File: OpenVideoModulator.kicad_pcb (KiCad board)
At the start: 2 copper layers, 38.6 x 24.9 mm, 22 parts, among them J1 CONN_6, J2 S-Video+Composite_Combo, P1 OSHW_LOGO, U1 AD724, Y1 4.433619M

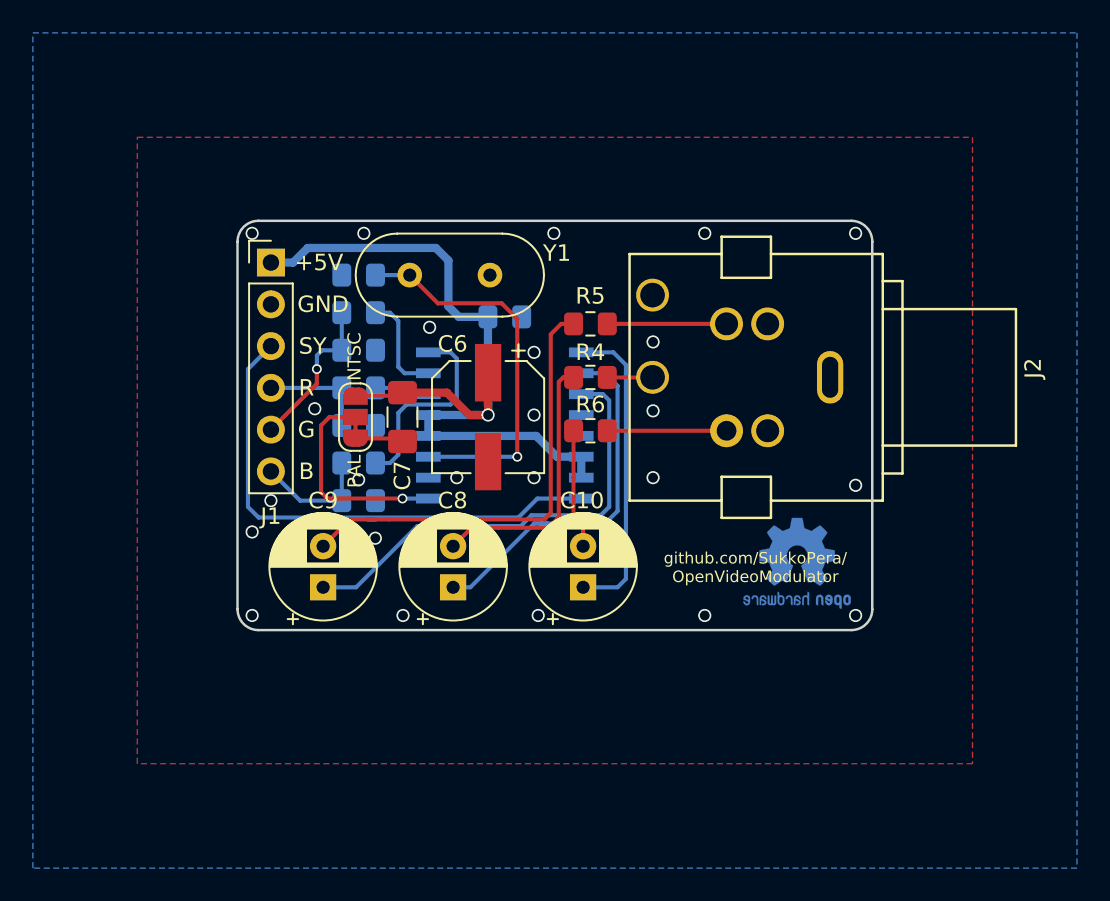
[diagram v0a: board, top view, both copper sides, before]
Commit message: 1st version
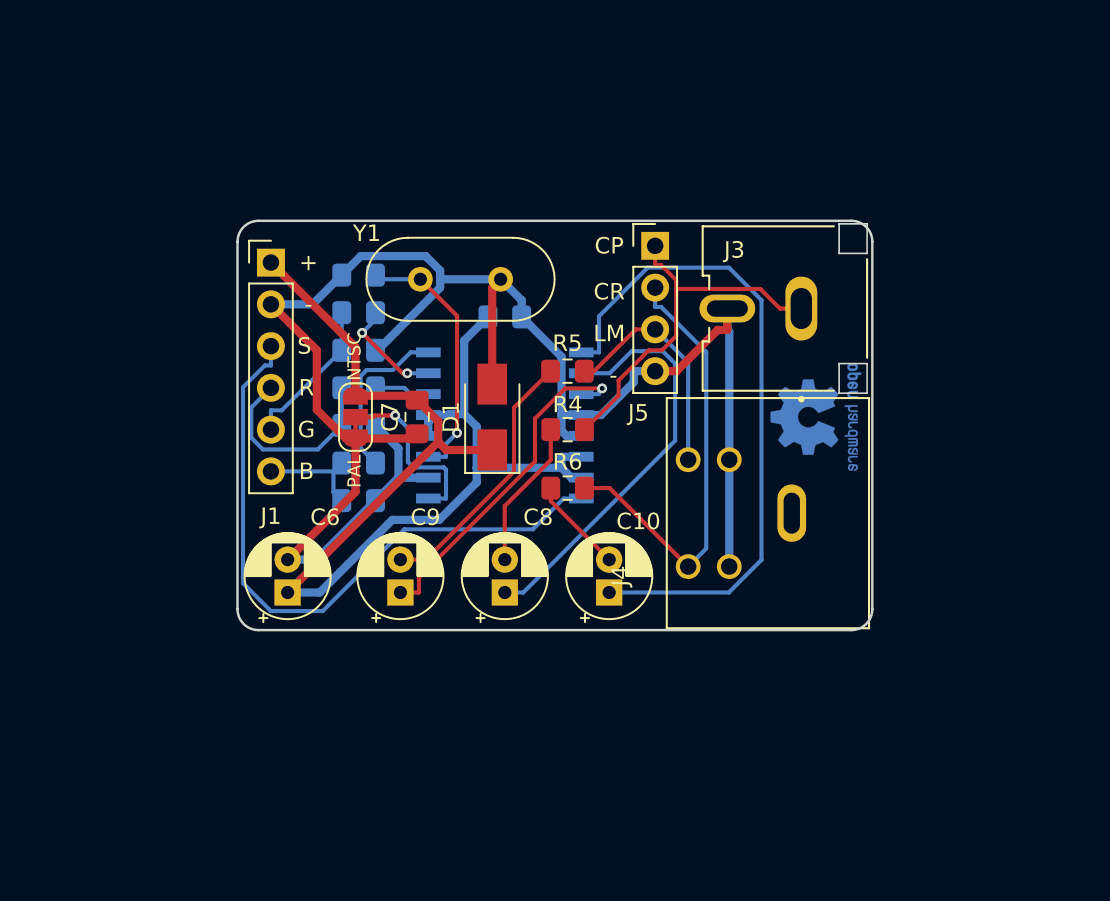
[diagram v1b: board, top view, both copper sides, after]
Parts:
- removed J2: S-Video+Composite_Combo, OpenVideoModulator:AV-MDC-401
- added D1: 1N4001, Diode_SMD:D_SMA, F.Cu at (129.5, 61.5)
- added J3: RCA, OpenVideoModulator:CUI_RCJ-044, F.Cu at (148.3, 54.9)
- added J4: Mini-DIN-4, OpenVideoModulator:CUI_MD-40S_1234, F.Cu at (146.3, 67.3)
- added J5: Conn_01x04_Male, Connector_PinHeader_2.54mm:PinHeader_1x04_P2.54mm_Vertical, F.Cu at (139.4, 51.1)
- C10, C8, C9: footprint Capacitor_THT:CP_Radial_D6.3mm_P2.50mm -> Capacitor_THT:CP_Radial_D5.0mm_P2.00mm
- C6: footprint Capacitor_SMD:CP_Elec_6.3x5.8 -> Capacitor_THT:CP_Radial_D5.0mm_P2.00mm
- C7: footprint Capacitor_SMD:C_1206_3216Metric_Pad1.42x1.75mm_HandSolder -> Capacitor_SMD:C_0805_2012Metric_Pad1.15x1.40mm_HandSolder
- moved C6 16.2 mm to (117.1, 72.1), turned to 90 degrees
- moved P1 8.96 mm to (149.2, 61.5), turned to 270 degrees
- moved C9 4.71 mm to (124.0, 72.1)
- moved R6 3.75 mm to (134.1, 65.8)
- moved R4 3.47 mm to (134.1, 62.2)
- moved R5 3.20 mm to (134.1, 58.7)
- moved C8 3.16 mm to (130.3, 72.1)
- moved C10 1.62 mm to (136.7, 72.1)
- moved C7 0.89 mm to (125.0, 61.5)
- moved Y1 0.70 mm to (130.0, 53.1)
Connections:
- R4 pad 1: Net-(J2-Pad6) -> COMP
- R5 pad 1: Net-(J2-Pad3) -> LUMA
- R6 pad 1: Net-(J2-Pad4) -> CRMA
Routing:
- net GND: track 2.94 -> 108.4 mm, vias 26 -> 0
- net CRMA: track 0.00 -> 27.2 mm
- net COMP: track 0.00 -> 22.8 mm
- net Net-(C10-Pad1): track 18.9 -> 41.1 mm
- net VAA: track 50.8 -> 71.0 mm, vias 1 -> 0
- net LUMA: track 0.00 -> 14.1 mm
- net Net-(C9-Pad2): track 27.7 -> 16.2 mm
- net /sync_in: track 31.4 -> 39.4 mm
- net Net-(C1-Pad1): track 23.9 -> 15.9 mm
- net Net-(C8-Pad2): track 16.4 -> 9.06 mm
- net Net-(J2-Pad4): track 7.25 -> 0.00 mm
- net Net-(J2-Pad3): track 7.25 -> 0.00 mm
- net Net-(C9-Pad1): track 27.8 -> 21.0 mm, vias 0 -> 1
- net /red_in: track 6.59 -> 12.2 mm
- net Net-(C8-Pad1): track 22.5 -> 25.5 mm
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- removed copper zone on B.Cu, net GND
- removed copper zone on F.Cu, net GND
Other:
- board text added: "+"
- board text added: "-"
- board text added: "CP"
- board text added: "CR"
- board text added: "LM"
- board text added: "S"
- board text added: "github.com/issalig/OpenVideoModulator"
- board text removed: "+5V"
- board text removed: "GND"
- board text removed: "SY"
- board text removed: "github.com/SukkoPera/ OpenVideoModulator"

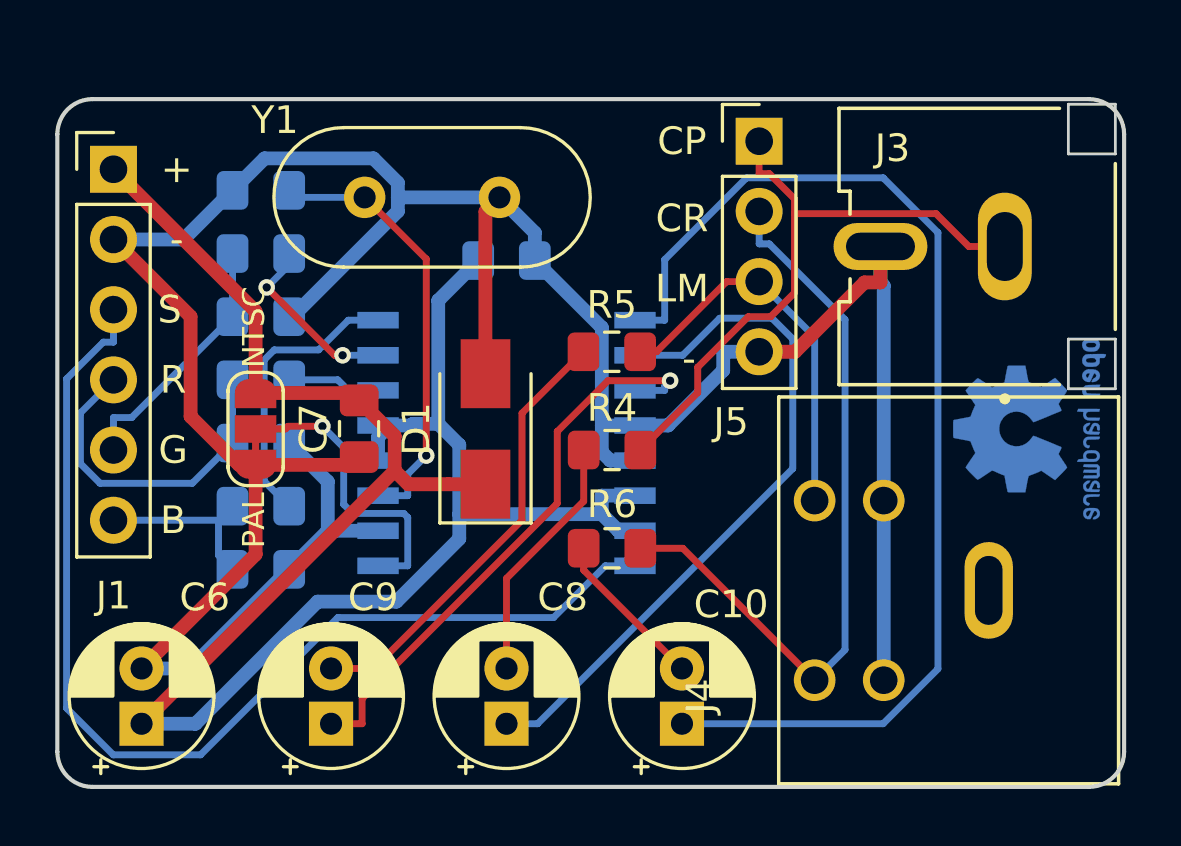
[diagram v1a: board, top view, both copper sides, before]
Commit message: panelizing experiments
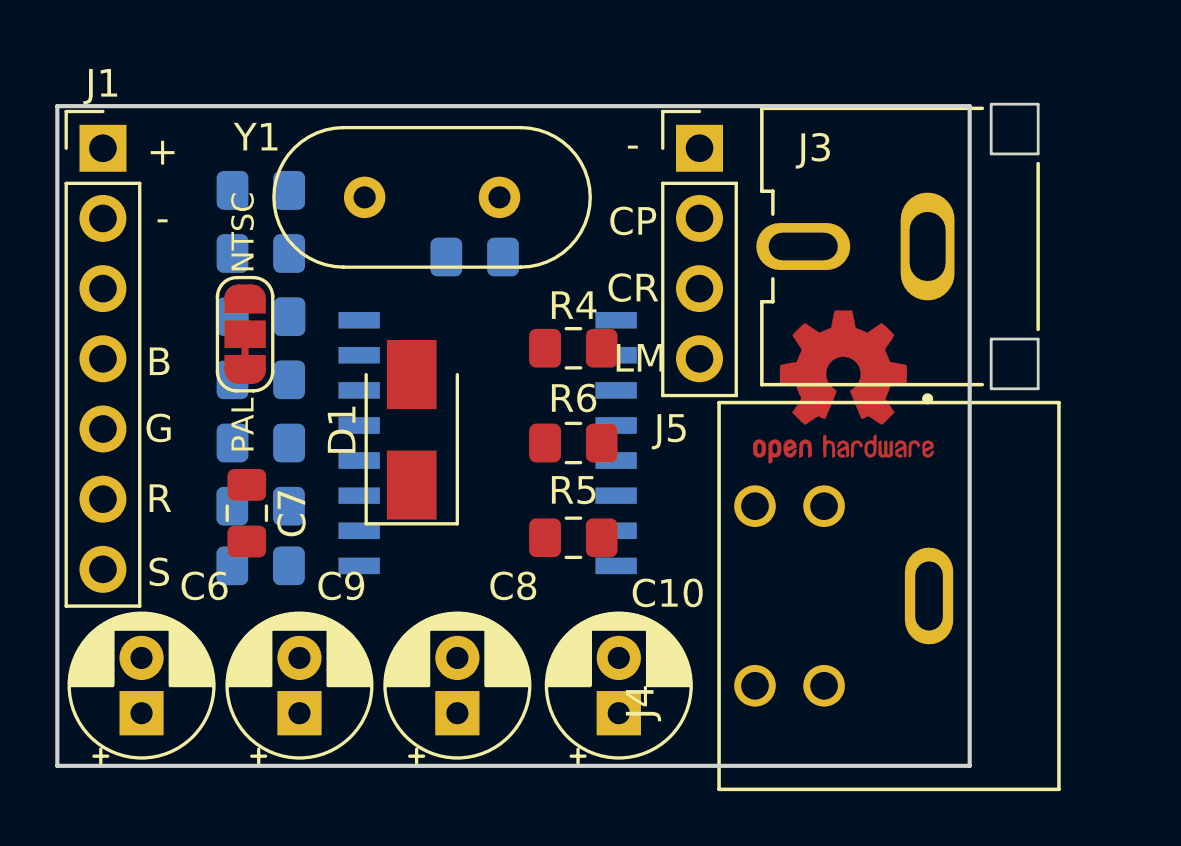
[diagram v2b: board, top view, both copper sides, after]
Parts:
- J1: value CONN_6 -> CONN_7; footprint Connector_PinHeader_2.54mm:PinHeader_1x06_P2.54mm_Vertical -> Connector_PinHeader_2.54mm:PinHeader_1x07_P2.54mm_Vertical
- P1: moved to F.Cu
- moved R3 9.14 mm to (121.4, 57.4)
- moved C4 9.14 mm to (121.4, 55.1)
- moved P1 6.90 mm to (142.5, 59.9), turned to 0 degrees
- moved R5 6.87 mm to (132.7, 65.4)
- moved C7 5.09 mm to (120.9, 64.5), turned to 270 degrees
- moved C2 4.57 mm to (121.4, 64.3)
- moved C3 4.57 mm to (121.4, 59.7)
- moved R2 4.57 mm to (121.4, 62.0)
- moved R1 4.45 mm to (121.4, 66.4)
- moved R6 4.06 mm to (132.7, 62.0)
- moved R4 3.94 mm to (132.7, 58.5)
- moved JP1 3.45 mm to (120.8, 58.0)
- moved J3 2.79 mm to (145.5, 54.9)
- moved D1 2.67 mm to (126.9, 61.5)
- moved C10 2.32 mm to (134.4, 71.8)
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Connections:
- J1 pad 3: /sync_in -> Net-(J1-Pad3)
- J1 pad 4: /red_in -> /blue_in
- J1 pad 6: /blue_in -> /red_in
- J5 pad 1: COMP -> GND
- J5 pad 2: CRMA -> COMP
- J5 pad 3: LUMA -> CRMA
- J5 pad 4: GND -> LUMA
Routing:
- net GND: track 108.4 -> 0.00 mm
- net VAA: track 71.0 -> 0.00 mm
- net Net-(C10-Pad1): track 41.1 -> 0.00 mm
- net /sync_in: track 39.4 -> 0.00 mm
- net CRMA: track 27.2 -> 0.00 mm
- net Net-(C8-Pad1): track 25.5 -> 0.00 mm
- net COMP: track 22.8 -> 0.00 mm
- net Net-(C9-Pad1): track 21.0 -> 0.00 mm, vias 1 -> 0
- net Net-(C9-Pad2): track 16.2 -> 0.00 mm
- net Net-(C1-Pad1): track 15.9 -> 0.00 mm, vias 1 -> 0
- net LUMA: track 14.1 -> 0.00 mm
- net /red_in: track 12.2 -> 0.00 mm
- net Net-(JP1-Pad2): track 10.9 -> 0.00 mm, vias 1 -> 0
- net Net-(C4-Pad1): track 10.4 -> 0.00 mm
- net /green_in: track 9.28 -> 0.00 mm
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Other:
- board size 38.6 x 24.9 mm -> 33 x 23.9 mm
- board text added: "Rev:0.1"
- board text added: "github.com/issalig/ OpenVideoModulator"
- board text removed: "V1"
- board text removed: "github.com/issalig/OpenVideoModulator"

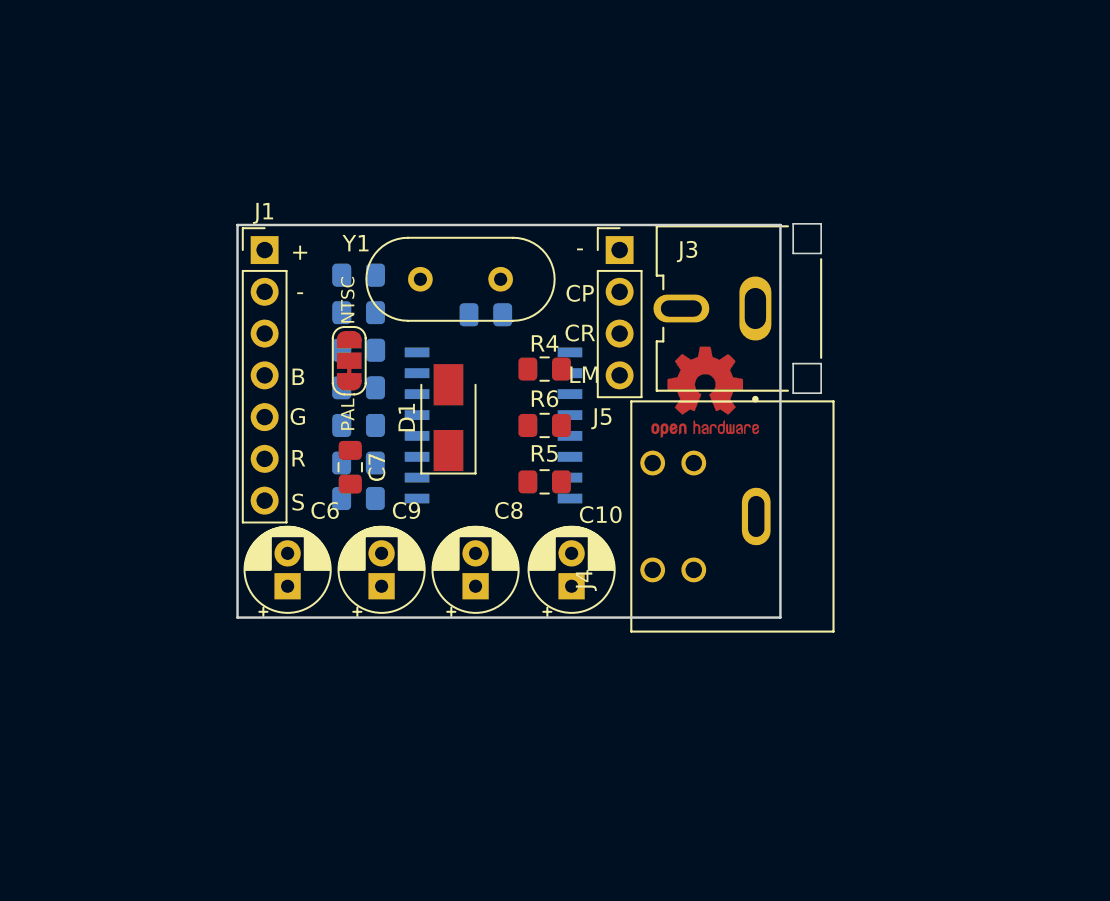
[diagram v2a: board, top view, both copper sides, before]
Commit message: release candidate
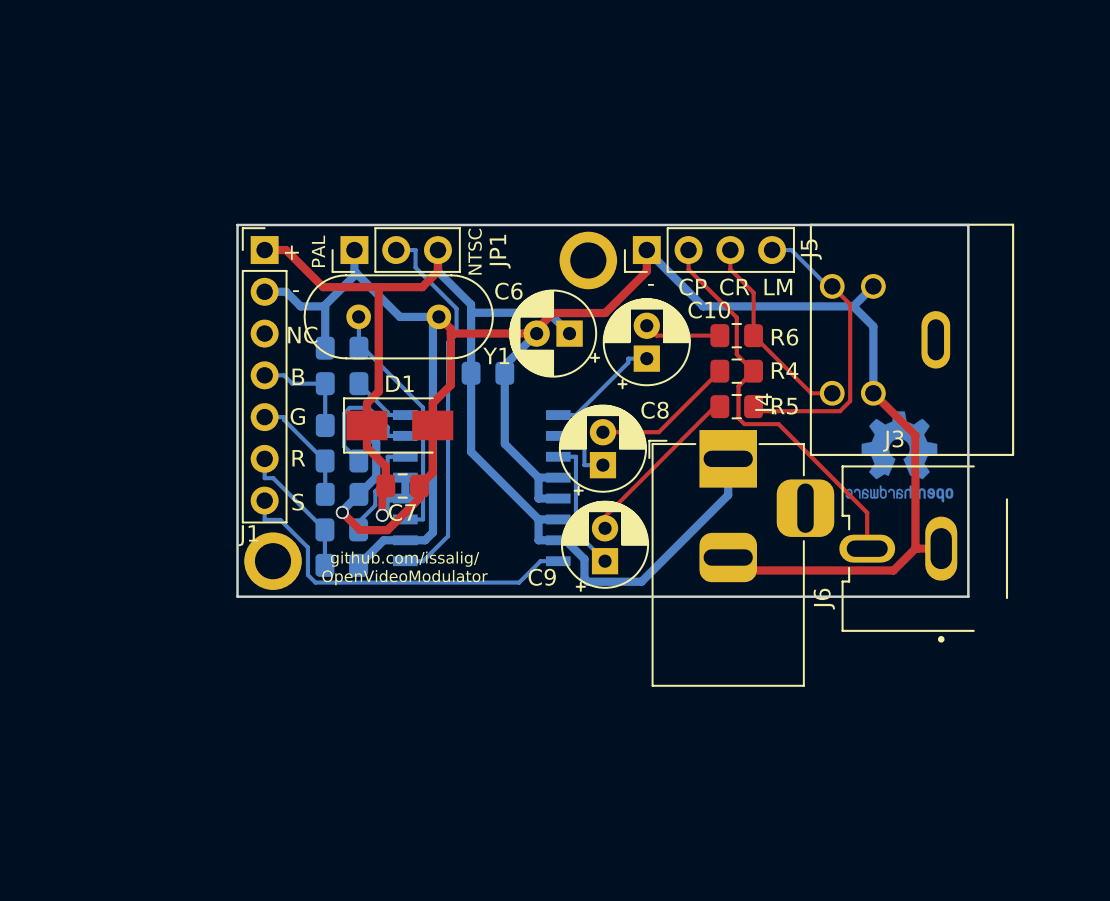
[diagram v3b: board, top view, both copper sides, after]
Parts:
- added H1: MountingHole, MountingHole:MountingHole_2.2mm_M2_ISO7380_Pad, F.Cu at (116.2, 70.2)
- added H2: MountingHole, MountingHole:MountingHole_2.2mm_M2_ISO7380_Pad, F.Cu at (135.4, 51.9)
- added J6: Barrel_Jack, Connector_BarrelJack:BarrelJack_Horizontal, F.Cu at (143.9, 64.0)
- JP1: footprint OpenVideoModulator:SolderJumper-3_P1.3mm_Bridged12_RoundedPad1.0x1.5mm -> Connector_PinHeader_2.54mm:PinHeader_1x03_P2.54mm_Vertical
- P1: moved to B.Cu
- moved C6 23.0 mm to (134.2, 56.4), turned to 180 degrees
- moved J3 18.5 mm to (156.8, 69.5)
- moved J4 15.3 mm to (155.1, 56.8)
- moved C10 14.6 mm to (138.9, 57.9)
- moved C9 13.7 mm to (136.4, 70.2)
- moved R6 12.9 mm to (144.4, 56.5)
- moved R5 12.5 mm to (144.4, 60.8)
- moved P1 12.4 mm to (154.3, 63.9), turned to 180 degrees
- moved R4 11.7 mm to (144.4, 58.7)
- moved C8 10.7 mm to (136.3, 64.4)
- moved JP1 6.74 mm to (121.2, 51.3)
- moved R3 4.68 mm to (120.4, 62.0)
- moved C3 4.56 mm to (120.4, 64.1)
- moved C1 4.56 mm to (120.4, 57.3)
- moved C4 4.43 mm to (120.4, 59.4)
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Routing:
- net GND: track 0.00 -> 134.9 mm, vias 0 -> 1
- net VAA: track 0.00 -> 77.0 mm, vias 0 -> 1
- net COMP: track 0.00 -> 24.6 mm
- net Net-(JP1-Pad2): track 0.00 -> 23.1 mm
- net /sync_in: track 0.00 -> 22.1 mm
- net LUMA: track 0.00 -> 18.2 mm
- net Net-(C1-Pad1): track 0.00 -> 15.2 mm
- net CRMA: track 0.00 -> 12.0 mm
- net Net-(C9-Pad2): track 0.00 -> 10.5 mm
- net Net-(C8-Pad2): track 0.00 -> 8.65 mm
- net /red_in: track 0.00 -> 8.30 mm
- net Net-(C9-Pad1): track 0.00 -> 8.16 mm
- net Net-(C3-Pad1): track 0.00 -> 8.14 mm
- net Net-(C10-Pad1): track 0.00 -> 6.95 mm
- net /green_in: track 0.00 -> 6.91 mm
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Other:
- board size 33 x 23.9 mm -> 44.5 x 22.6 mm
- board text added: "Designed with KiCad"
- board text added: "JLCJLCJLCJLC"
- board text added: "Licensed under CERN OHL v.2.0"
- board text added: "NC"
- board text added: "issalig 03/2021 Rev:0.1"
- board text removed: "Licensed under CERN OHL v.1.2"
- board text removed: "Rev:0.1"
